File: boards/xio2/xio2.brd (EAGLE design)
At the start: 170 x 100 mm, 376 parts, among them J1 12401598E4#2A, Q1 BSS138, Q2 BSS138, Q3 BC817-16LT3G, Q4 BC817-16LT3G, Y2 FA-238 25.0000MB-K3

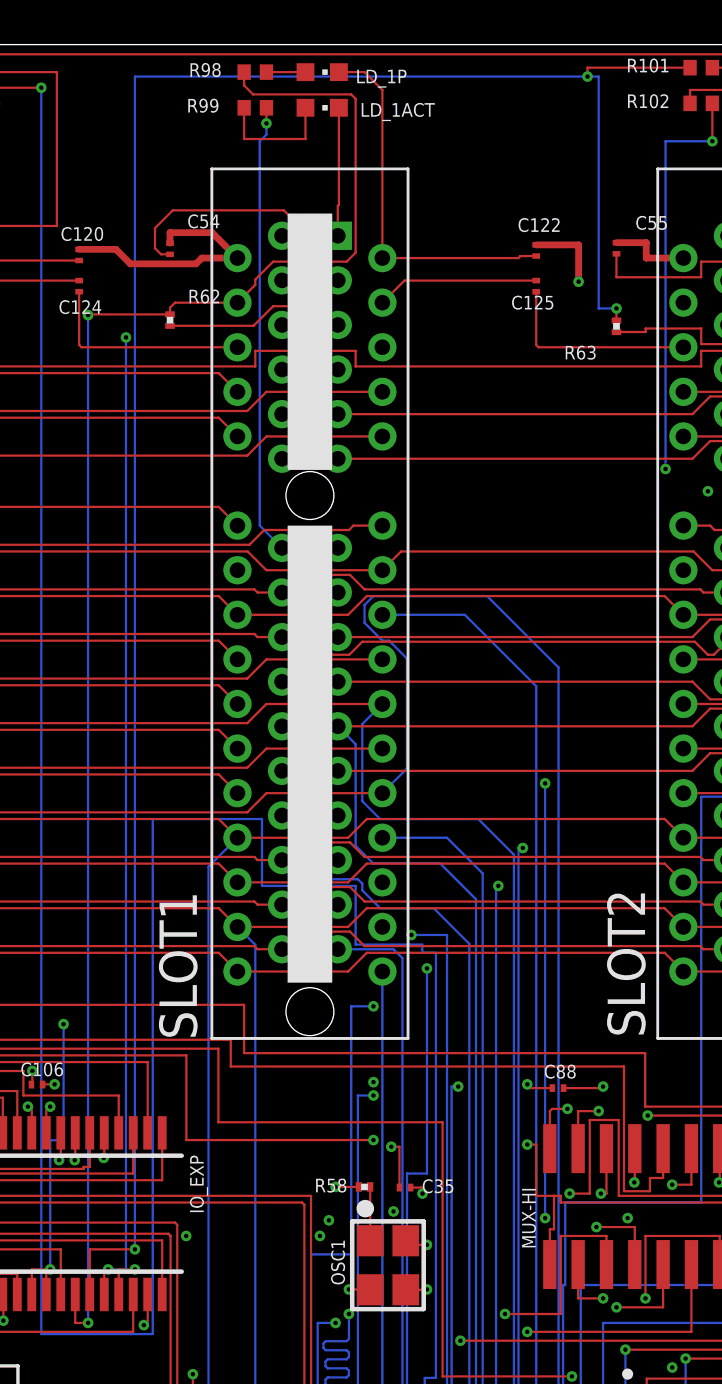
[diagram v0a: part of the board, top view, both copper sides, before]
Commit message: Text changes
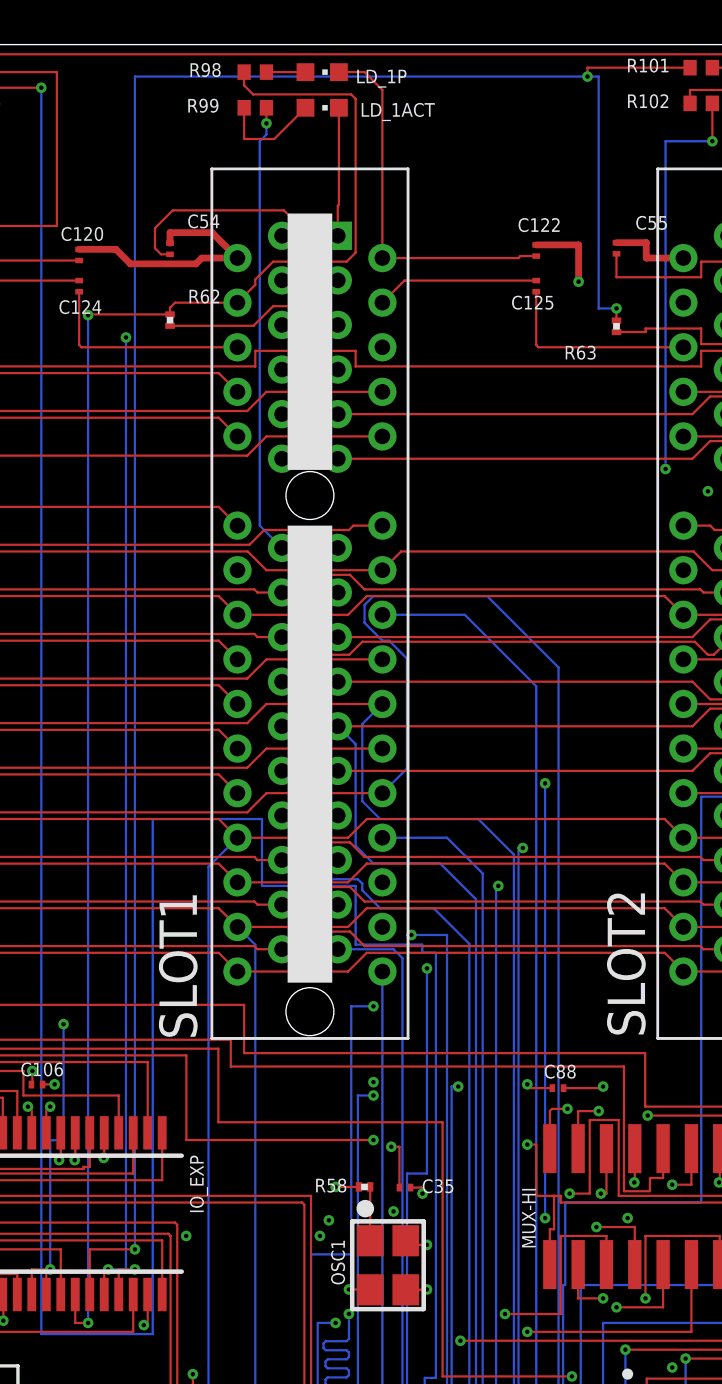
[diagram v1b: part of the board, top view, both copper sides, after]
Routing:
- net SPI_IRQ2: track 114.6 -> 111.0 mm
- net N$92: track 5.55 -> 4.73 mm
- net SPI_SS1: track 112.0 -> 111.3 mm
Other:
- board text added: "Silkscreen needs work Space for version label"
- board text removed: "Silkscreen needs work SDRAM ought to be length-matched QSPI ought to be length-matched SD Card ought to be length-matched Space for version label"
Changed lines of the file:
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@@
 <setting verticaltext="up"/>
 </settings>
-<grid distance="0.1" unitdist="mm" unit="mm" style="lines" multiple="1" display="yes" altdistance="1" altunitdist="mil" altunit="mil"/>
+<grid distance="1" unitdist="mil" unit="mil" style="lines" multiple="1" display="yes" altdistance="1" altunitdist="mil" altunit="mil"/>
 <layers>
 <layer number="1" name="Top" color="4" fill="1" visible="yes" active="yes"/>
@@
 <text x="152.6" y="15.6" locked="yes" size="0.6096" layer="25">+5V @ 10A
 Center +VE</text>
-<text x="71.05" y="-14.2" locked="yes" size="0.6096" layer="50">Silkscreen needs work
-SDRAM ought to be length-matched
-QSPI ought to be length-matched
-SD Card ought to be length-matched
+<text x="77.55" y="-11.5" size="0.6096" layer="50">Silkscreen needs work
 Space for version label</text>
 </plain>
@@
 <wire x1="25.5" y1="60.3" x2="25.5" y2="85.1" width="0.1016" layer="16"/>
 <wire x1="25.5" y1="85.1" x2="24.9" y2="85.1" width="0.1016" layer="16"/>
-<wire x1="78.3" y1="97.1" x2="78.3" y2="96.2" width="0.1016" layer="3"/>
-<wire x1="78.3" y1="96.2" x2="38.8" y2="96.2" width="0.1016" layer="3"/>
+<wire x1="78.3" y1="97.1" x2="78.3" y2="96.2127" width="0.1016" layer="3"/>
+<wire x1="78.3" y1="96.2127" x2="78.2873" y2="96.2" width="0.1016" layer="3" curve="-90"/>
+<wire x1="78.2873" y1="96.2" x2="38.8" y2="96.2" width="0.1016" layer="3"/>
 <wire x1="38.8" y1="96.2" x2="38.8" y2="86.4" width="0.1016" layer="3"/>
-<wire x1="38.8" y1="86.4" x2="24.9" y2="86.4" width="0.1016" layer="3"/>
-<wire x1="24.9" y1="86.4" x2="24.9" y2="85.1" width="0.1016" layer="3"/>
 <wire x1="78.3" y1="97.1" x2="78.3" y2="97.8" width="0.1016" layer="1"/>
 <wire x1="25.1" y1="60.3" x2="25.5" y2="59.9" width="0.1016" layer="1"/>
@@
 <via x="78.3" y="97.1" extent="1-16" drill="0.2" diameter="0.4794"/>
 <via x="25.1" y="60.3" extent="1-16" drill="0.2" diameter="0.4794"/>
+<wire x1="38.8" y1="86.4" x2="26.2" y2="86.4" width="0.1016" layer="3"/>
+<wire x1="26.2" y1="86.4" x2="24.9" y2="85.1" width="0.1016" layer="3"/>
 </signal>
 <signal name="SPI_SS2" class="11">
@@
 <wire x1="90.8" y1="47.2" x2="90.8" y2="48" width="0.1016" layer="3"/>
 <wire x1="90.8" y1="67.5" x2="90.8" y2="48" width="0.1016" layer="16"/>
-<wire x1="90.8" y1="67.5" x2="90.8" y2="77.06" width="0.1016" layer="14"/>
-<wire x1="90.8" y1="77.06" x2="97" y2="77.06" width="0.1016" layer="14"/>
 <wire x1="81" y1="36" x2="81.5" y2="35.5" width="0.1016" layer="1"/>
 <wire x1="37.9" y1="54.7" x2="37.5" y2="55.1" width="0.1016" layer="1"/>
@@
 <via x="81" y="36" extent="1-16" drill="0.2" diameter="0.4794"/>
 <via x="37.9" y="54.7" extent="1-16" drill="0.2" diameter="0.4794"/>
+<wire x1="90.8" y1="67.5" x2="90.8" y2="70.86" width="0.1016" layer="14"/>
+<wire x1="90.8" y1="70.86" x2="97" y2="77.06" width="0.1016" layer="14"/>
 </signal>
 <signal name="SPI_IRQ3" class="11">
@@
 <wire x1="92.7" y1="99.2" x2="92.7" y2="99.6" width="0.1016" layer="1"/>
 <wire x1="92.7" y1="99.6" x2="97.3" y2="99.6" width="0.1016" layer="1"/>
-<wire x1="72.4" y1="46.6" x2="72.4" y2="99.2" width="0.1016" layer="16"/>
-<wire x1="72.4" y1="99.2" x2="92.7" y2="99.2" width="0.1016" layer="16"/>
+<wire x1="72.4" y1="46.6" x2="72.4" y2="99.1873" width="0.1016" layer="16"/>
+<wire x1="72.4" y1="99.1873" x2="72.4127" y2="99.2" width="0.1016" layer="16" curve="-90"/>
+<wire x1="72.4127" y1="99.2" x2="92.7" y2="99.2" width="0.1016" layer="16"/>
 <wire x1="92.7" y1="99.2" x2="93.2" y2="99.2" width="0.1016" layer="16"/>
 <wire x1="72.4" y1="46.6" x2="70.375" y2="46.6" width="0.1016" layer="1"/>
@@
 <contactref element="LD_1ACT" pad="A"/>
 <wire x1="77.3" y1="97.8" x2="77.3" y2="96.4" width="0.1016" layer="1"/>
-<wire x1="77.3" y1="96.4" x2="80.05" y2="96.4" width="0.1016" layer="1"/>
-<wire x1="80.05" y1="96.4" x2="80.05" y2="97.8" width="0.1016" layer="1"/>
+<wire x1="77.3" y1="96.4" x2="78.65" y2="96.4" width="0.1016" layer="1"/>
+<wire x1="78.65" y1="96.4" x2="80.05" y2="97.8" width="0.1016" layer="1"/>
 </signal>
 <signal name="N$94">

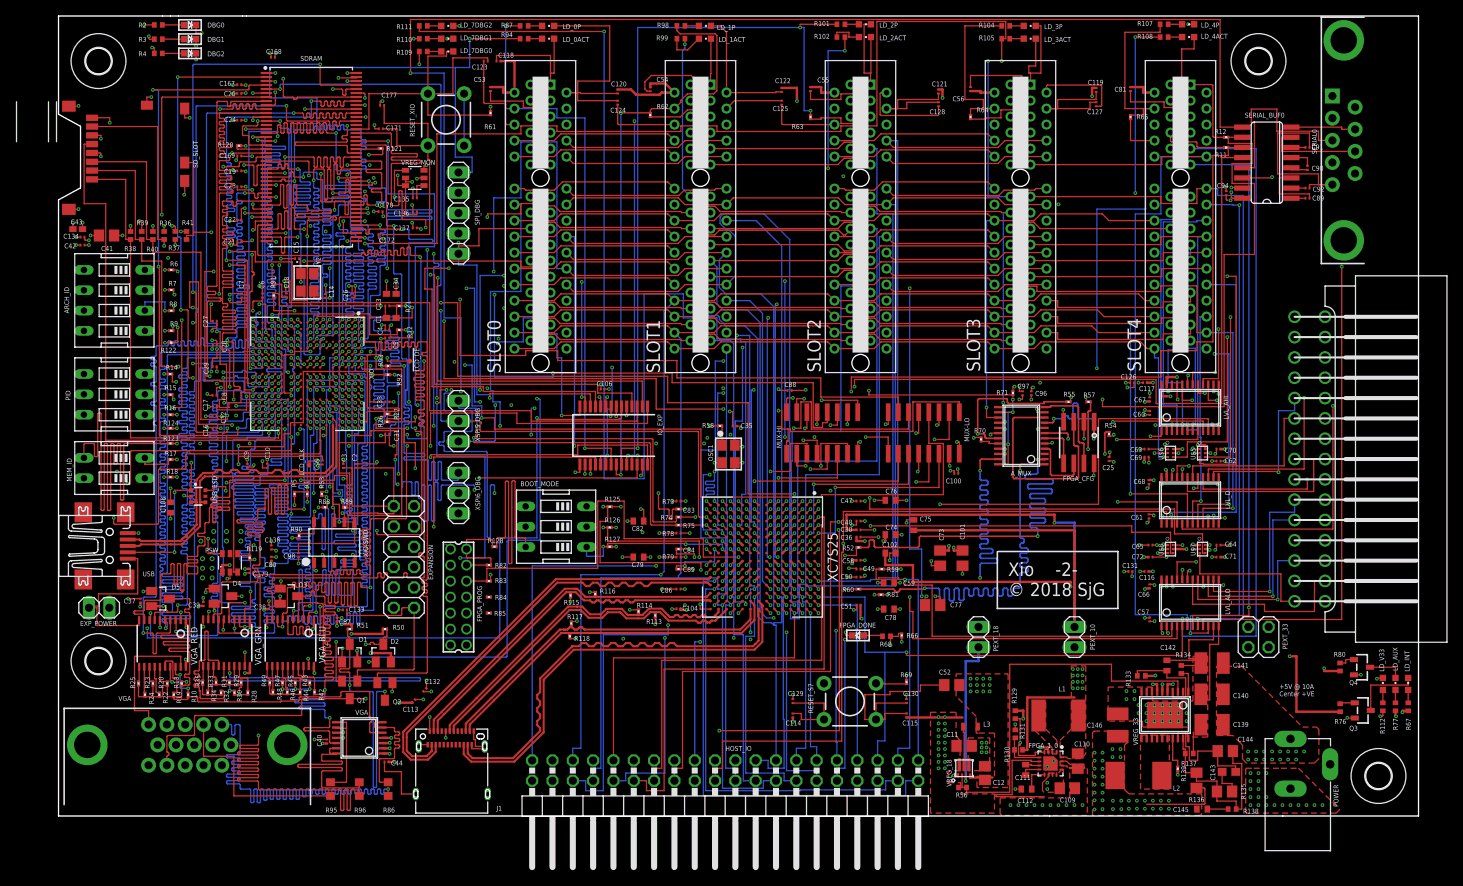
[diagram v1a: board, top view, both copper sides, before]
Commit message: Checkpoint
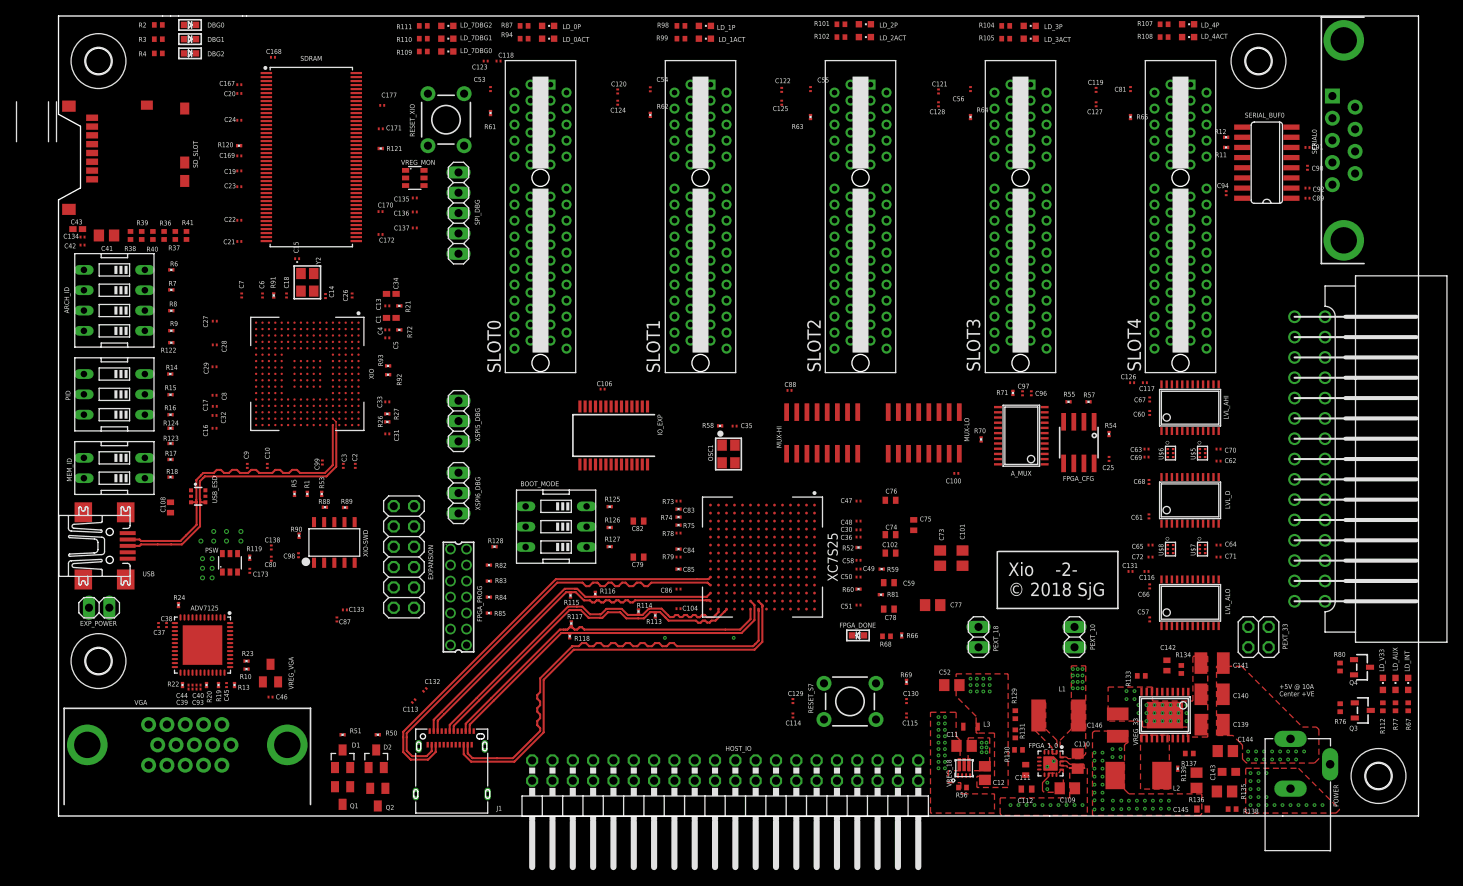
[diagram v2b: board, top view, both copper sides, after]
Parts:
- removed !LCD_DE!, LCD_CLK: PTR1TP06R, testpad:TP06R
- removed D3, D4, D5: BAT54S, diode:SOT23
- removed R25, R35, R49: 549R, rcl:R0201
- removed R28, R42: 71.5K, rcl:R0201
- removed R29, R43: 35.7K, rcl:R0201
- removed R30, R44: 17.8K, rcl:R0201
- removed R31, R45: 8.66K, rcl:R0201
- removed R32, R46: 4.32K, rcl:R0201
- removed R33, R47: 2.21K, rcl:R0201
- removed R34, R48: 1.05K, rcl:R0201
- removed R86, R95, R96: 68R, rcl:R0603
- removed VGA_: MAX4382, sjg-opamp:TSSOP14
- removed VGA_BLU, VGA_GRN, VGA_RED: (no value), microbuilder:TSSOP20
- added ADV7125: ADV7125, sjg-analog:QFN50P700X700X100-49T495
- added C45: 0.1uF, rcl:C0201
- added C46: 1uF, rcl:C0201
- added C93: 0.01uF, rcl:C0201
- added VREG_VGA: AD1580ARTZ, sjg-analog:SOT23
- C37, C44: value 0.1uF -> 0.01uF
- R10: value 71.5K -> 560R
- R13: value 35.7K -> 1K
- R19: value 17.8K -> 75R
- R20: value 8.66K -> 75R
- R22: value 4.32K -> 75R
- R23: value 2.21K -> 4.7K
- R24: value 1.05K -> 0R
- moved C44 26.3 mm to (16.5, 17.0)
- moved C40 17.5 mm to (17.5, 17.0), turned to 0 degrees
- moved D1 13.2 mm to (35.5, 7.79)
- moved D2 13.2 mm to (39.7, 7.79)
- moved R50 13.2 mm to (39.9, 10.8)
- moved R51 13.2 mm to (35.5, 10.8)
- moved Q1 13.2 mm to (35.5, 3.19)
- moved Q2 13.2 mm to (39.9, 2.99)
- moved C38 13.0 mm to (13.5, 24.5), turned to 270 degrees
- moved R23 12.0 mm to (23.5, 20.0), turned to 0 degrees
- moved R24 12.0 mm to (15.0, 27.0), turned to 270 degrees
- moved C39 10.8 mm to (16.5, 16.5), turned to 180 degrees
- moved R10 7.97 mm to (23.5, 19.0), turned to 180 degrees
- moved R13 6.60 mm to (22.0, 17.0), turned to 270 degrees
- moved R19 5.73 mm to (20.0, 17.0)
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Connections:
- removed net LCDCLK: LCD_CLK.TP, XIO.F16
- removed net N$20: R22.2, VGA_RED.14
- removed net N$21: R23.2, VGA_RED.13
- removed net N$22: R24.2, VGA_RED.12
- removed net N$23: R25.2, VGA_RED.11
- removed net N$24: R35.2, VGA_GRN.11
- removed net N$25: R86.1, VGA_.6, VGA_.7
- removed net N$26: R34.2, VGA_GRN.12
- removed net N$27: R33.2, VGA_GRN.13
- removed net N$34: R32.2, VGA_GRN.14
- removed net N$35: R31.2, VGA_GRN.15
- removed net N$36: R30.2, VGA_GRN.16
- removed net N$37: R95.2, VGA.2
- removed net N$38: R29.2, VGA_GRN.17
- removed net N$39: R28.2, VGA_GRN.18
- removed net N$40: R49.2, VGA_BLU.11
- removed net N$41: R48.2, VGA_BLU.12
- removed net N$42: R47.2, VGA_BLU.13
- removed net N$43: R46.2, VGA_BLU.14
- removed net N$44: R45.2, VGA_BLU.15
- removed net N$45: R44.2, VGA_BLU.16
- removed net N$46: R43.2, VGA_BLU.17
- removed net N$47: R42.2, VGA_BLU.18
- removed net N$53: !LCD_DE!.TP, XIO.D7
- removed net VGA_BLUE: D3.3, R42.1, R43.1, R44.1, R45.1, R46.1, R47.1, R48.1, R49.1, VGA_.12
- removed net VGA_GRN: D4.3, R28.1, R29.1, R30.1, R31.1, R32.1, R33.1, R34.1, R35.1, VGA_.10
- removed net VGA_RED: D5.3, R10.1, R13.1, R19.1, R20.1, R22.1, R23.1, R24.1, R25.1, VGA_.5
- new net LCD_BLANK: ADV7125.11, XIO.D7
- new net LCD_CLK: ADV7125.24, XIO.F16
- net +3V3: now also ADV7125.13, ADV7125.29, ADV7125.30, C37.1, C38.1, C39.1, C40.1, C44.1, C45.1, C93.1, R13.2, R23.2
- net +5V: no longer C37.1, C38.1, C39.1, C40.1, C44.1, D3.2, D4.2, D5.2, VGA_.1, VGA_.2, VGA_.3, VGA_.4, VGA_BLU.1, VGA_BLU.20, VGA_GRN.1, VGA_GRN.20, VGA_RED.1, VGA_RED.20
- net GND: now also ADV7125.1, ADV7125.14, ADV7125.15, ADV7125.2, ADV7125.25, ADV7125.26, ADV7125.27, ADV7125.31, ADV7125.33, ADV7125.39, ADV7125.40, ADV7125.49, C46.2, C93.2, R10.1, R19.2, R20.2, R22.2, R24.1, VREG_VGA.2; no longer D3.1, D4.1, D5.1, VGA_.11, VGA_BLU.10, VGA_BLU.19, VGA_GRN.10, VGA_GRN.19, VGA_RED.10, VGA_RED.19
- net LCD_B0: now also ADV7125.16; no longer VGA_BLU.2
- net LCD_B1: now also ADV7125.17; no longer VGA_BLU.3
- net LCD_B2: now also ADV7125.18; no longer VGA_BLU.4
- net LCD_B3: now also ADV7125.19; no longer VGA_BLU.5
- net LCD_B4: now also ADV7125.20; no longer VGA_BLU.6
- net LCD_B5: now also ADV7125.21; no longer VGA_BLU.7
- net LCD_B6: now also ADV7125.22; no longer VGA_BLU.8
- net LCD_B7: now also ADV7125.23; no longer VGA_BLU.9
- net LCD_G0: now also ADV7125.3; no longer VGA_GRN.2
- net LCD_G1: now also ADV7125.4; no longer VGA_GRN.3
- net LCD_G2: now also ADV7125.5; no longer VGA_GRN.4
- net LCD_G3: now also ADV7125.6; no longer VGA_GRN.5
- net LCD_G4: now also ADV7125.7; no longer VGA_GRN.6
- net LCD_G5: now also ADV7125.8; no longer VGA_GRN.7
- net LCD_G6: now also ADV7125.9; no longer VGA_GRN.8
- net LCD_G7: now also ADV7125.10; no longer VGA_GRN.9
- net LCD_R0: now also ADV7125.41; no longer VGA_RED.2
- net LCD_R1: now also ADV7125.42; no longer VGA_RED.3
- net LCD_R2: now also ADV7125.43; no longer VGA_RED.4
- net LCD_R3: now also ADV7125.44; no longer VGA_RED.5
- net LCD_R4: now also ADV7125.45; no longer VGA_RED.6
- net LCD_R5: now also ADV7125.46; no longer VGA_RED.7
- net LCD_R6: now also ADV7125.47; no longer VGA_RED.8
- net LCD_R7: now also ADV7125.48; no longer VGA_RED.9
- net N$10: now also ADV7125.38, R23.1; no longer R96.2, VGA.3
- net N$17: now also ADV7125.37, R10.2; no longer R19.2, VGA_RED.16
- net N$18: now also ADV7125.12, R24.2; no longer R20.2, VGA_RED.15
- net N$6: now also ADV7125.36, C46.1, R13.1, VREG_VGA.1; no longer R10.2, VGA_RED.18
- net N$8: now also ADV7125.35, C45.2; no longer R13.2, VGA_RED.17
- net VGA_B: now also ADV7125.28, R22.1, VGA.3; no longer R96.1, VGA_.13, VGA_.14
- net VGA_G: now also ADV7125.32, R20.1, VGA.2; no longer R95.1, VGA_.8, VGA_.9
- net VGA_R: now also ADV7125.34, R19.1; no longer R86.2
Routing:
- net GND: track 799.5 -> 0.00 mm, vias 353 -> 62
- net HOST_A2: track 302.7 -> 0.00 mm, vias 4 -> 0
- net HOST_A6: track 301.8 -> 0.00 mm, vias 5 -> 0
- net +3V3: track 300.2 -> 0.00 mm, vias 213 -> 36
- net HOST_A0: track 296.5 -> 0.00 mm, vias 4 -> 0
- net HOST_A7: track 295.8 -> 0.00 mm, vias 4 -> 0
- net HOST_A1: track 295.6 -> 0.00 mm, vias 3 -> 0
- net HOST_A10: track 288.2 -> 0.00 mm, vias 4 -> 0
- net HOST_A4: track 285.4 -> 0.00 mm, vias 5 -> 0
- net HOST_A3: track 282.9 -> 0.00 mm, vias 3 -> 0
- net HOST_A14: track 281.6 -> 0.00 mm, vias 6 -> 0
- net HOST_A5: track 268.1 -> 0.00 mm, vias 5 -> 0
- net HOST_A11: track 266.0 -> 0.00 mm, vias 7 -> 0
- net HOST_A15: track 261.9 -> 0.00 mm, vias 5 -> 0
- net HOST_A12: track 252.5 -> 0.00 mm, vias 5 -> 0
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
